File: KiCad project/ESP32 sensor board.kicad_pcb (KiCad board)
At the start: 4 copper layers, 103 x 53 mm, 87 parts, among them J1 USB_C_Receptacle, J2 JST_2mm_LiPo, J3 GSD090012SEU, J4 B4B-XH-AM, J6 Conn_01x05, Q1 TEMT6000X01, Q2 BC817, Q3 BC817, SW1 1101NE, SW2 1101NE, U1 MCP73871, U2 LM1117MPX-3.3_NOPB, U3 ESP32-C3-WROOM-02-H4, U4 CP2102N-A02-GQFN20, U5 USBLC6-2SC6, U6 W25Q32JVSSIQ, U7 BME280, U8 MAX4466EXK+T

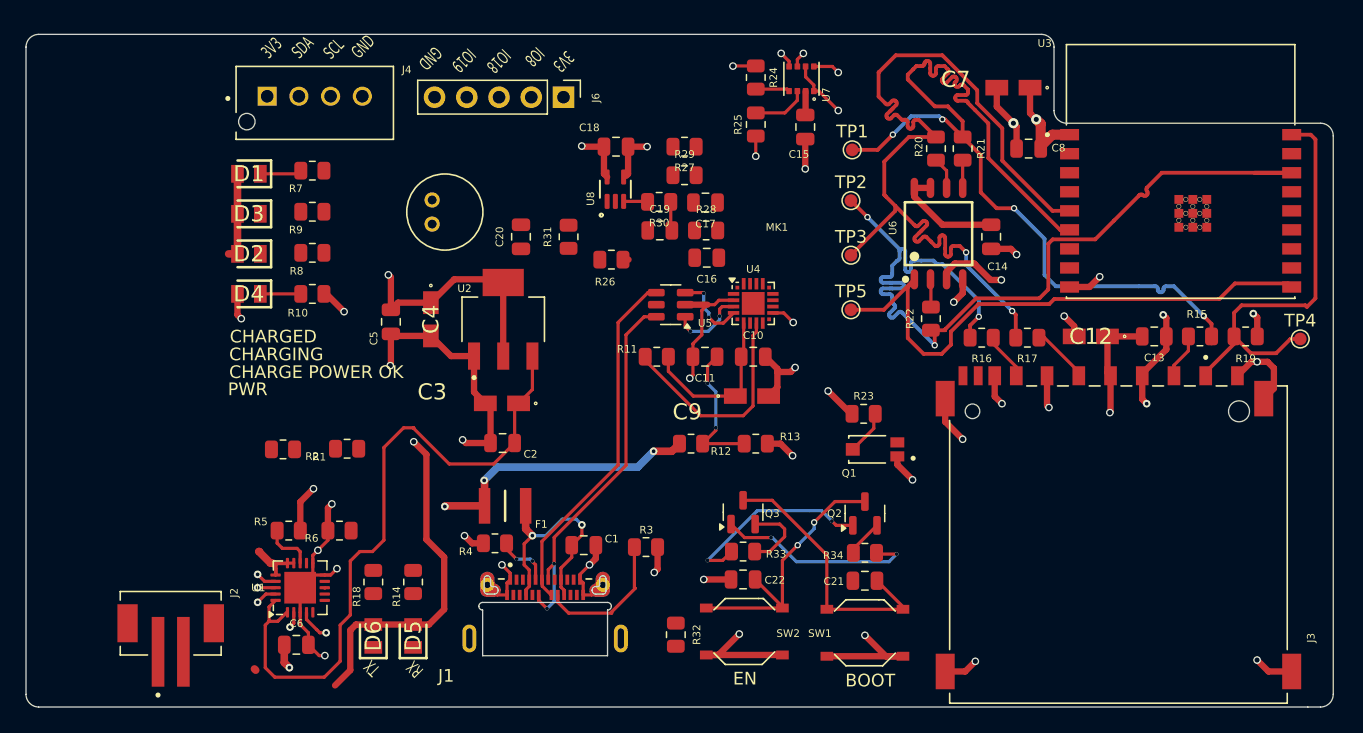
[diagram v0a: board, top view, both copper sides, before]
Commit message: Completed layout for v2.
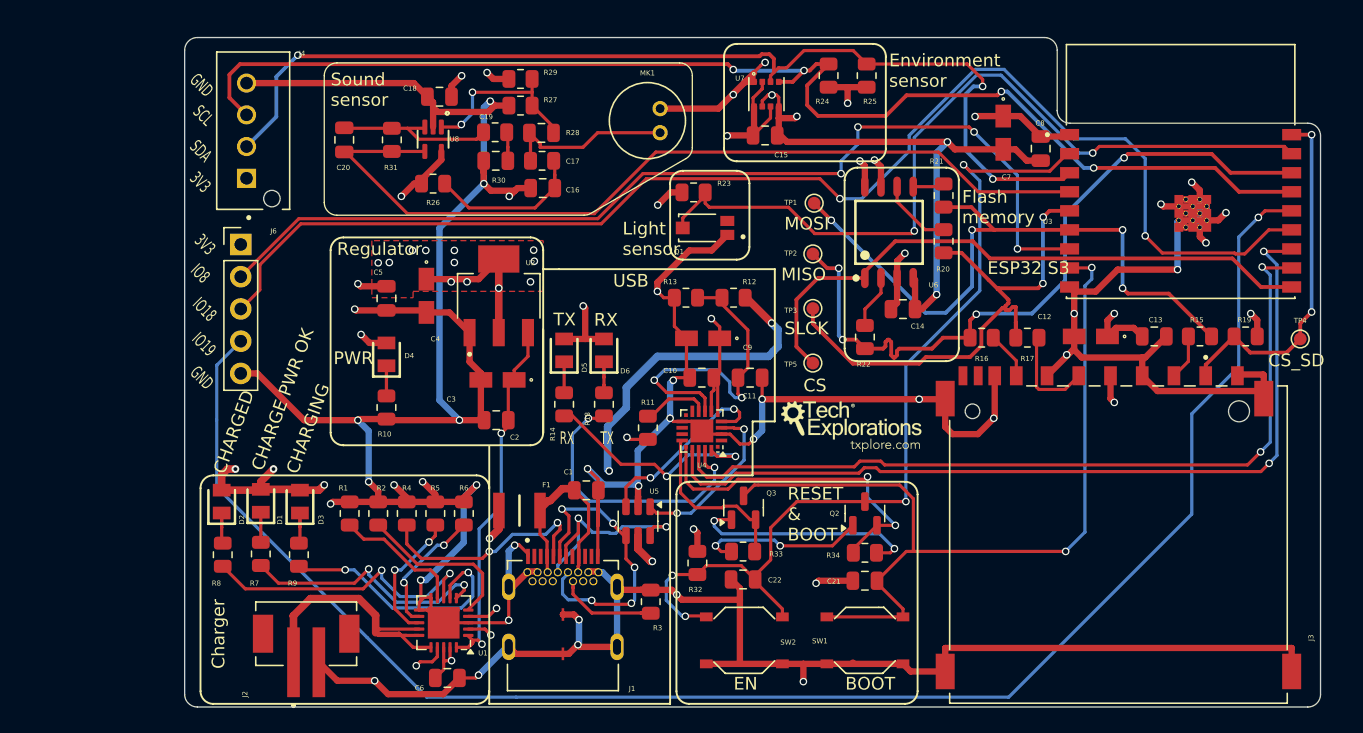
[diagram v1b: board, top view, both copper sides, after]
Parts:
- added G***: LOGO, Footprints:TE_Logo_11.6x4, F.Cu at (163.0, 102.8)
- J1: footprint Footprints:TE_1-2295018-2 -> Footprints:BELFUSE_SS-52400-002
- moved R7 30.5 mm to (116.5, 112.9), turned to 90 degrees
- moved D6 28.9 mm to (143.5, 96.9)
- moved J6 28.0 mm to (114.9, 88.6), turned to 0 degrees
- moved R9 27.0 mm to (119.5, 113.0), turned to 90 degrees
- moved D1 25.8 mm to (116.5, 108.8), turned to 90 degrees
- moved D5 25.5 mm to (140.4, 96.9)
- moved R8 24.8 mm to (113.5, 113.0), turned to 90 degrees
- moved D3 23.0 mm to (119.6, 108.8), turned to 90 degrees
- moved R18 22.9 mm to (143.5, 101.2)
- moved Q1 22.0 mm to (151.5, 87.2)
- moved R23 22.0 mm to (150.6, 84.5)
- moved D2 19.6 mm to (113.4, 108.8), turned to 90 degrees
- moved R14 18.4 mm to (140.4, 101.2)
- moved MK1 17.5 mm to (147.0, 78.8), turned to 0 degrees
- moved U5 17.3 mm to (146.2, 110.4), turned to -90 degrees
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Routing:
- net GND: track 156.1 -> 473.5 mm, vias 37 -> 43
- net /ESP32-C3-02/GPIO19: track 0.00 -> 130.3 mm, vias 0 -> 1
- net /ESP32-C3-02/GPIO18: track 0.00 -> 104.2 mm, vias 0 -> 2
- net /ESP32-C3-02/SCL: track 2.69 -> 101.0 mm, vias 0 -> 4
- net /ESP32-C3-02/GPIO8: track 0.00 -> 78.9 mm, vias 0 -> 4
- net /ESP32-C3-02/SDA: track 4.41 -> 83.2 mm, vias 0 -> 3
- net /ESP32-C3-02/MIC_OUT: track 0.00 -> 68.7 mm
- net /ESP32-C3-02/RX_TX: track 0.00 -> 68.4 mm, vias 0 -> 2
- net /ESP32-C3-02/TX_RX: track 0.00 -> 64.6 mm, vias 0 -> 2
- net /ESP32-C3-02/PHOTO_C: track 3.54 -> 63.4 mm, vias 0 -> 2
- net /ESP32-C3-02/EN: track 21.6 -> 71.7 mm, vias 2 -> 4
- net /ESP32-C3-02/BOOT: track 21.8 -> 68.8 mm, vias 0 -> 2
- net /ESP32-C3-02/SCLK: track 69.0 -> 43.6 mm
- net /ESP32-C3-02/MOSI_DI: track 75.4 -> 51.1 mm
- net /ESP32-C3-02/RTS: track 2.93 -> 26.8 mm, vias 0 -> 2
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- added copper zone on In2.Cu, net /+5V_USB
- added copper zone on F.Cu, net 3.3V
- added copper zone on In2.Cu, net GND
- removed copper zone on In2.Cu, net 3.3V
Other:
- board size 103 x 53 mm -> 89.5 x 52.8 mm
- board text added: "CHARGE PWR OK"
- board text added: "CS"
- board text added: "CS_SD"
- board text added: "Charger"
- board text added: "ESP32 S3"
- board text added: "Environment sensor"
- board text added: "Flash memory"
- board text added: "Light sensor"
- board text added: "MISO"
- board text added: "MOSI"
- board text added: "RESET & BOOT"
- board text added: "Regulator"
- board text added: "SLCK"
- board text added: "Sound sensor"
- board text added: "USB"
- board text removed: "CHARGE POWER OK"
